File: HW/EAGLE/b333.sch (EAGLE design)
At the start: 153 parts, among them Q1 BF423, Q5 NMOSD, X2 USB MICRO

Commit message: .
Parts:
- added 1C13, C10, C9: 100n, resistor:C-EUC0805
- added 1C6: 1n, resistor:C-EUC0805K
- added 1C7, 3C13, C17, C18: 100n, resistor:C-EUC0805K
- added 1C8, 1C9: 22p, resistor:C-EUC0805K
- added 1L2: 10mkhn, rcl:L-USIRF-24
- added 1R10, 1R9: 10K, resistor:R-EU_R0805
- added 1R17: 3K3, resistor:R-EU_R1206W
- added 1R18: 27K, resistor:R-EU_R0805
- added 1R19, 1R21, 1R23: 680, resistor:R-EU_0207/10
- added 1R20, 1R22, 1R24: 470K, resistor:R-EU_0207/10
- added 1R25: 2K2, resistor:R-EU_R0805
- added 1R26: 270, resistor:R-EU_R1206W
- added 1RC2: 22K, resistor:R-EU_R0805
- added 1RC2*1: 4K3, resistor:R-EU_R1206W
- added 1Z2: 8MHz, crystal:CRYSTALHC49U70
- added 3C12: 47u, resistor:CPOL-EUE2.5-6
- added 4R6, 4R7: 100, resistor:R-EU_R0805
- added 4Y3, 4Y4: РЭС55А, relay_ussr:РЭС55А
- added D7: MEGA328P-AU, avr-6:MEGA48/88/168-AU
- added D8: TL431, v-reg:TL431CLP
- added DA6: 78L05, v-reg:78LXX
- added H2: LCD, pinhead:PINHD-1X16
- added ISP: (no value), con-lstb:MA03-2
- added J_NO_LI, J_ONE5V: (no value), jumper:SJ
- added R14: 180K, resistor:R-EU_R0805
- added R15: 20.0k, resistor:R-EU_R0805
- added R16: 180.0k, resistor:R-EU_R0805
- added R4: 20K, resistor:R-EU_R0805
- added T4, T5, T6: (no value), pinhead:PINHD-1X1
- added TEST1: TT-P, transistor_tester:TT-P
- R24: device resistor:R-EU_R0805 -> resistor:R-EU_0204/7
- renumbered X2 to X1
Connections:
- net N$57 renamed +40V
- new net +5V/2: 1R26.2, 1RC2.1, 3C12.+, C18.1, DA6.OUT, H2.2, J_ONE5V.2
- new net E1: D7.PD5(T1/OC0B/PCINT21), H2.6
- new net N$60: 1RC2*1.2, 1RC2.2, H2.3
- new net N$61: 1R26.1, H2.15
- new net N$62: D7.PD3(INT1/OC2B/PCINT19), H2.14
- new net N$63: R14.2
- new net N$64: 1C6.1, D7.AREF
- new net N$68: 1C8.2, 1Z2.2, D7.PB6(XTAL1/TOSC1/PCINT6)
- new net N$69: 1C9.2, 1Z2.1, D7.PB7(XTAL2/TOSC2/PCINT7)
- new net N$70: 1C13.1, 1L2.1, D7.AVCC
- new net N$71: 4R6.2, 4Y3G$2.P
- new net N$72: 4R7.2, 4Y4G$2.P
- new net N$87: D7.PD0(RXD/PCINT16), H2.11
- new net N$88: D7.PD1(TXD/PCINT17), H2.12
- new net N$89: D7.PD2(INT0/PCINT18), H2.13
- new net PB3: 1R19.1, D7.PB0(ICP1/CLKO/PCINT0)
- new net PB4: 1R20.1, D7.PB1(OC1A/PCINT1)
- new net PB5: 1R21.1, D7.PB2(SS/OC1B/PCINT2)
- new net PC10: 1R21.2, 1R22.2, 4Y4G$2.O, D7.PC1(ADC1/PCINT9), T5.1, TEST1.2
- new net PC11: 1R23.2, 1R24.2, 4Y3G$2.O, D7.PC2(ADC2/PCINT10), T6.1, TEST1.3
- new net PC6: 1R10.2, 1R17.2, D7.PC5(ADC5/SCL/PCINT13)
- new net PC7: 1R25.2, D7.PC4(ADC4/SDA/PCINT12), D8.C, D8.R
- new net PC8: C9.1, D7.PC3(ADC3/PCINT11), R14.1, R4.2
- new net PC9: 1R19.2, 1R20.2, 4R6.1, 4R7.1, D7.PC0(ADC0/PCINT8), T4.1, TEST1.1
- new net PD1: 1R18.2, C17.1, D7.PD7(AIN1/PCINT23)
- new net PD2: D7.PD6(AIN0/OC0A/PCINT22)
- new net RS1: D7.PD4(T0/XCK/PCINT20), H2.4
- new net V+1: 1R10.1, 1R9.2
- net +5V: now also 1C7.1, 1L2.2, 1R18.1, 1R25.1, C10.1, D7.VCC@1, D7.VCC@2, ISP.2, J_NO_LI.2, J_ONE5V.1
- net +7V: now also DA6.IN, J_NO_LI.1
- net GND: now also 1C13.2, 1C6.2, 1C7.2, 1C8.1, 1C9.1, 1R17.1, 1RC2*1.1, 3C12.-, 3C13.2, C10.2, C17.2, C18.2, C9.2, D7.AGND, D7.GND@1, D7.GND@2, D8.A, DA6.GND, H2.1, H2.10, H2.16, H2.5, H2.7, H2.8, H2.9, ISP.6, R15.1, R4.1
- net MISO: now also 1R23.1, D7.PB4(MISO/PCINT4), ISP.1
- net MOSI: now also 1R22.1, D7.PB3(MOSI/OC2A/PCINT3), ISP.4
- net N$18: now also R16.2
- net PC3: now also 3C13.1, R15.2, R16.1
- net RESET: now also 1R9.1, D7.PC6(/RESET/PCINT14), ISP.5
- net SCK: now also 1R24.1, D7.PB5(SCK/PCINT5), ISP.3
- net UGND: now also DA1..

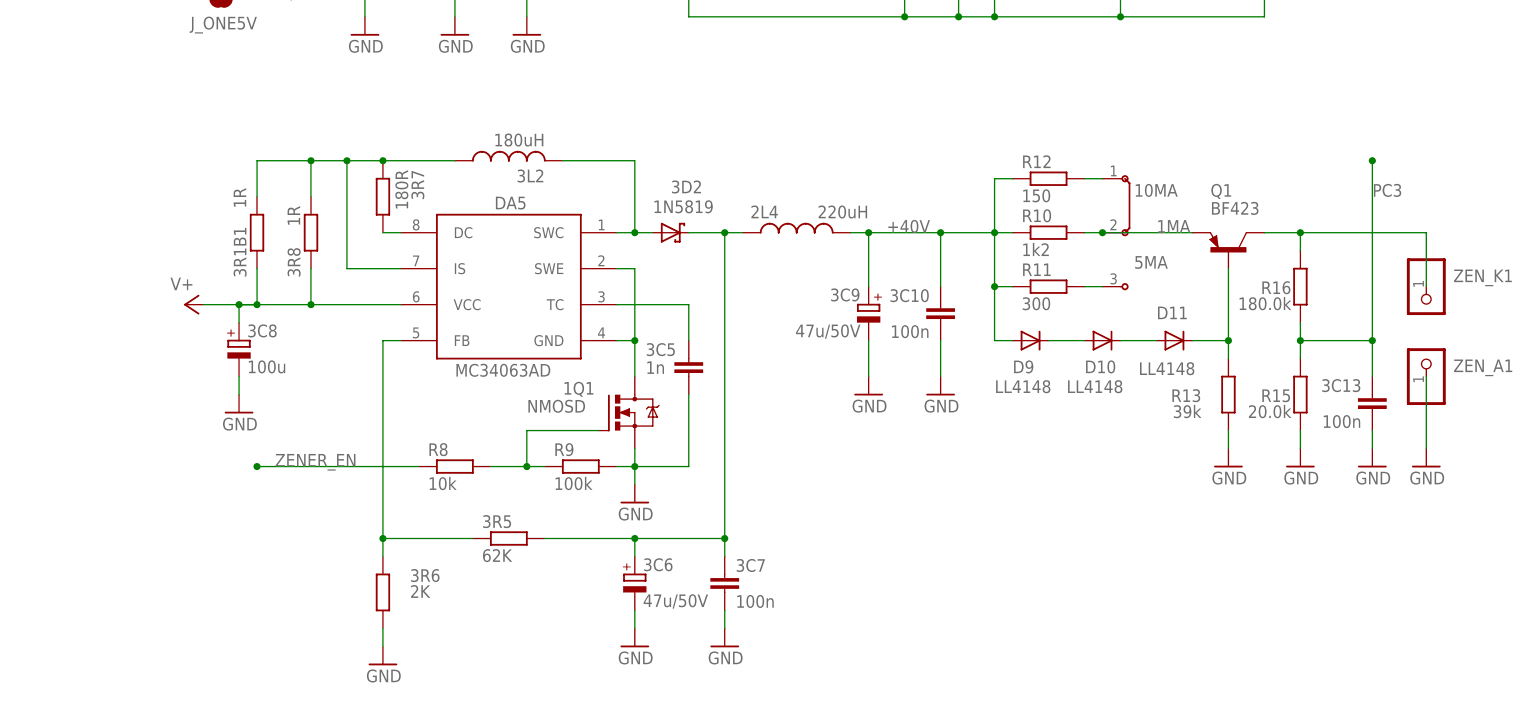
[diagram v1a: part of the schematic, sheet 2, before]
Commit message: .
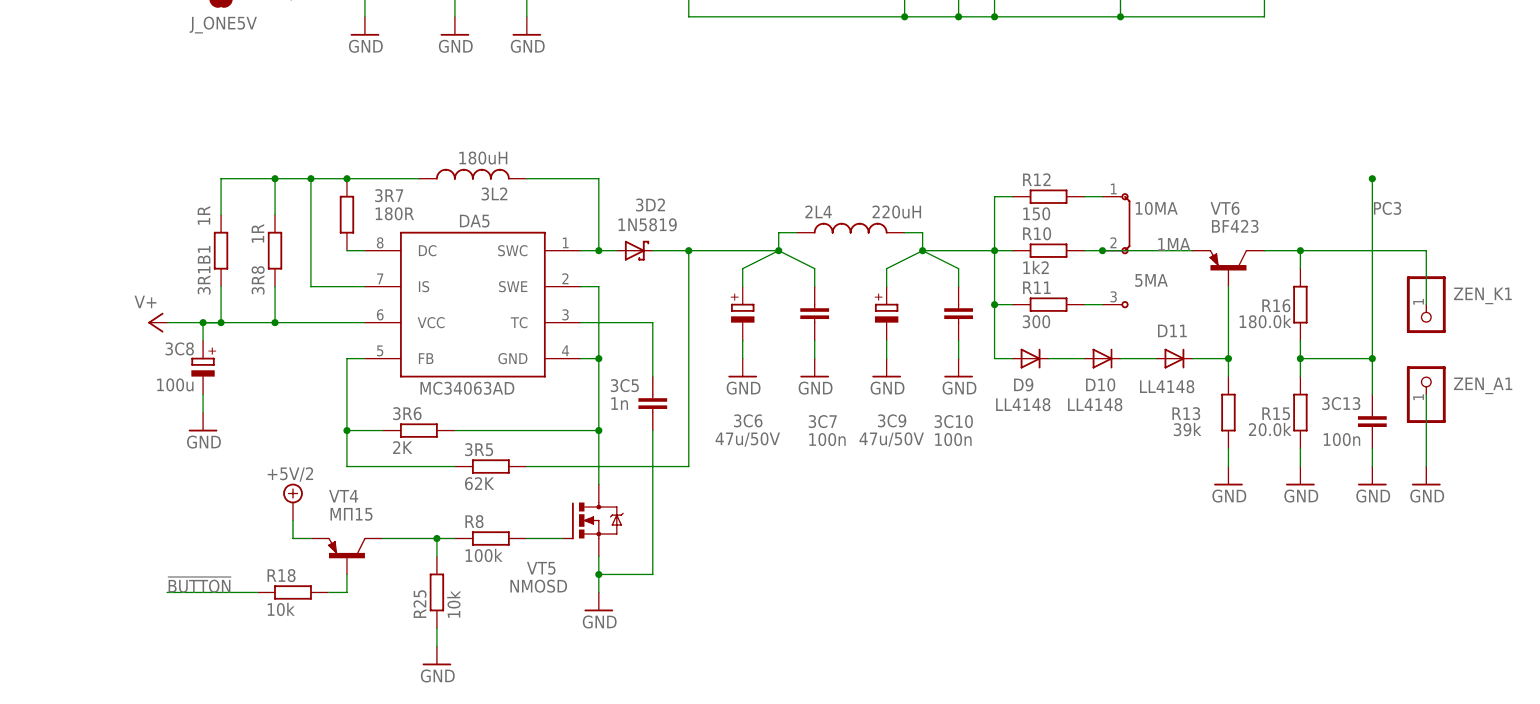
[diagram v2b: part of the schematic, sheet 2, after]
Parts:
- removed 1Q1: NMOSD, DSS:NMOSD
- removed Q1: BF423, transistor-pnp:BF423
- removed R9: 100k, resistor:R-EU_R0805
- added R18, R25: 10k, resistor:R-EU_R0805
- added VT4: МП15, transistor-pnp:BF423
- added VT5: NMOSD, DSS:NMOSD
- added VT6: BF423, transistor-pnp:BF423
- R8: value 10k -> 100k
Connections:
- removed net ZENER_EN: R8.1
- new net !BUTTON: R18.1
- new net N$73: R25.2, R8.1, VT4.C
- new net N$74: R18.2, VT4.B
- net +5V/2: now also VT4.E
- net 1MA: now also VT6.E; no longer Q1.E
- net GND: now also R25.1, VT5.S; no longer 1Q1.S, 3R6.2, R9.2
- net N$18: now also VT6.C; no longer Q1.C
- net N$56: now also VT5.G; no longer 1Q1.G, R9.1
- net N$58: now also 3R6.2, VT5.D; no longer 1Q1.D
- net N$67: now also VT6.B; no longer Q1.B
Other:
- moved on the sheet: 2L4, 3C10, 3C13, 3C5, 3C6, 3C7, 3C8, 3C9, 3D2, 3L2, 3R1B1, 3R5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
